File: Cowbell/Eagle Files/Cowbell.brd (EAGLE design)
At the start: 100 x 50 mm, 71 parts, among them IC1 LM741P, Q1 2N3906, T1 2N3904, T2 2N3904, T3 2N3904, T4 2N3904, T5 2N3904, T6 2N3904, T7 2N3904, T8 2N3904

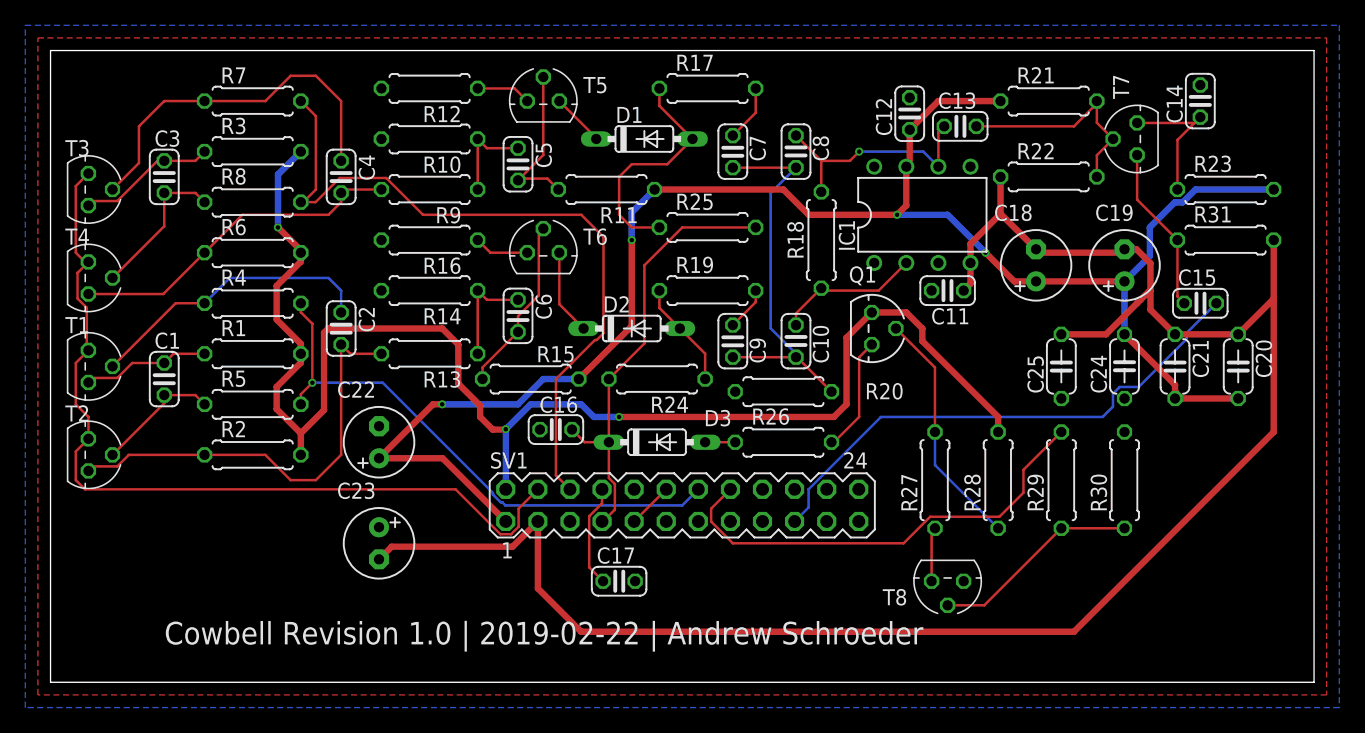
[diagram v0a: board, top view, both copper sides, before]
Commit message: cleanup
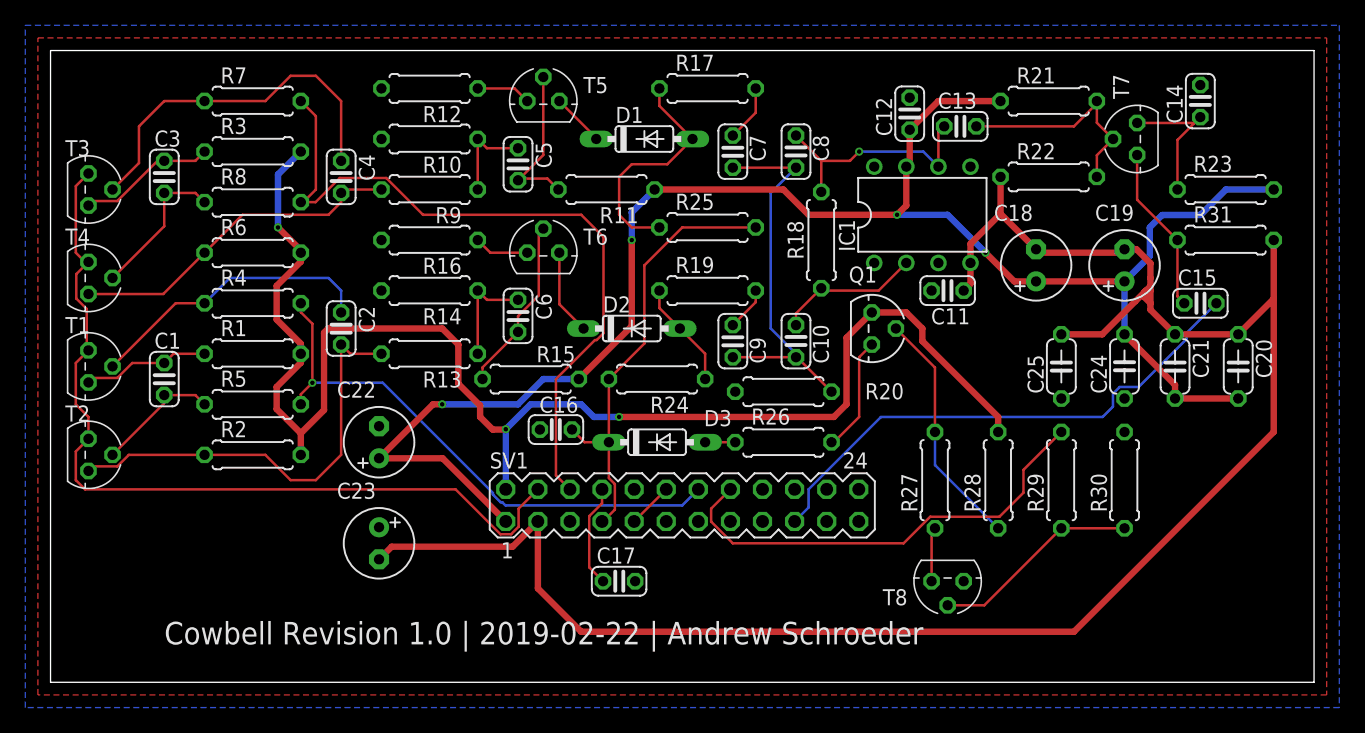
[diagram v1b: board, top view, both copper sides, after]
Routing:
- net -12V: track 148.5 -> 150.2 mm
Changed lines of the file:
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@@
 <?xml version="1.0" encoding="utf-8"?>
 <!DOCTYPE eagle SYSTEM "eagle.dtd">
-<eagle version="9.2.2">
+<eagle version="9.3.1">
 <drawing>
 <settings>
@@
 </class>
 </classes>
-<designrules name="JLCPCB2Layer">
+<designrules name="SeeedStudio_2layer_DRU_no_angle_20140221">
 <description language="de">&lt;b&gt;EAGLE Design Rules&lt;/b&gt;
 &lt;p&gt;
@@
 </description>
 <param name="layerSetup" value="(1*16)"/>
-<param name="mtCopper" value="0.035mm 0.035mm 0.035mm 0.035mm 0.035mm 0.035mm 0.035mm 0.035mm 0.035mm 0.035mm 0.035mm 0.035mm 0.035mm 0.035mm 0.035mm 0.035mm"/>
-<param name="mtIsolate" value="1.5mm 0.15mm 0.2mm 0.15mm 0.2mm 0.15mm 0.2mm 0.15mm 0.2mm 0.15mm 0.2mm 0.15mm 0.2mm 0.15mm 0.2mm"/>
+<param name="mtCopper" value="0.035mm 0.0175mm 0.035mm 0.035mm 0.035mm 0.035mm 0.035mm 0.035mm 0.035mm 0.035mm 0.035mm 0.035mm 0.035mm 0.035mm 0.0175mm 0.035mm"/>
+<param name="mtIsolate" value="1.5mm 1.1mm 0.2mm 0.15mm 0.2mm 0.15mm 0.2mm 0.15mm 0.2mm 0.15mm 0.2mm 0.15mm 0.2mm 0.15mm 0.2mm"/>
 <param name="mdWireWire" value="6mil"/>
 <param name="mdWirePad" value="6mil"/>
@@
 <param name="mdSmdStop" value="0mil"/>
 <param name="msWidth" value="6mil"/>
-<param name="msDrill" value="10mil"/>
-<param name="msMicroVia" value="10mil"/>
+<param name="msDrill" value="12mil"/>
+<param name="msMicroVia" value="12mil"/>
 <param name="msBlindViaRatio" value="0.5"/>
 <param name="rvPadTop" value="0.25"/>
@@
 <param name="rvMicroViaOuter" value="0.25"/>
 <param name="rvMicroViaInner" value="0.25"/>
-<param name="rlMinPadTop" value="6mil"/>
+<param name="rlMinPadTop" value="10mil"/>
 <param name="rlMaxPadTop" value="20mil"/>
-<param name="rlMinPadInner" value="6mil"/>
+<param name="rlMinPadInner" value="10mil"/>
 <param name="rlMaxPadInner" value="20mil"/>
-<param name="rlMinPadBottom" value="6mil"/>
+<param name="rlMinPadBottom" value="10mil"/>
 <param name="rlMaxPadBottom" value="20mil"/>
 <param name="rlMinViaOuter" value="6mil"/>
@@
 <wire x1="46" y1="37.19" x2="47.81" y2="39" width="0.508" layer="16"/>
 <wire x1="85" y1="31.73" x2="85" y2="27.54" width="0.508" layer="16"/>
-<wire x1="90.62684375" y1="39" x2="96.81" y2="39" width="0.508" layer="16"/>
+<wire x1="93.02684375" y1="39" x2="96.81" y2="39" width="0.508" layer="16"/>
 <wire x1="31.03" y1="17.73" x2="36.03" y2="12.73" width="0.508" layer="1"/>
 <wire x1="31.03" y1="17.73" x2="26" y2="17.73" width="0.508" layer="1"/>
@@
 <wire x1="85" y1="31.73" x2="87" y2="33.73" width="0.508" layer="16"/>
 <wire x1="87" y1="33.73" x2="87" y2="36" width="0.508" layer="16"/>
-<wire x1="87" y1="36" x2="88.984" y2="37.984" width="0.508" layer="16"/>
-<wire x1="88.984" y1="37.984" x2="89.61084375" y2="37.984" width="0.508" layer="16"/>
-<wire x1="89.61084375" y1="37.984" x2="90.62684375" y2="39" width="0.508" layer="16"/>
+<wire x1="87" y1="36" x2="87.984" y2="36.984" width="0.508" layer="16"/>
+<wire x1="87.984" y1="36.984" x2="91.01084375" y2="36.984" width="0.508" layer="16"/>
+<wire x1="91.01084375" y1="36.984" x2="93.02684375" y2="39" width="0.508" layer="16"/>
 </signal>
 <signal name="-12V">
@@
 <wire x1="89" y1="27.54" x2="87.0525" y2="29.4875" width="0.508" layer="1"/>
 <wire x1="85" y1="34" x2="85" y2="34.27" width="0.2" layer="1"/>
-<wire x1="87.0525" y1="29.4875" x2="87.0525" y2="31" width="0.508" layer="1"/>
-<wire x1="87.0525" y1="31" x2="87.0525" y2="33.1659625" width="0.508" layer="1"/>
+<wire x1="87.0525" y1="29.4875" x2="87.0525" y2="30" width="0.508" layer="1"/>
+<wire x1="87.0525" y1="30" x2="87.0525" y2="31" width="0.508" layer="1"/>
+<wire x1="87.0525" y1="31" x2="87.0525" y2="31.3525" width="0.508" layer="1"/>
+<wire x1="87.0525" y1="32" x2="87.0525" y2="33.1659625" width="0.508" layer="1"/>
 <wire x1="87.0525" y1="33.1659625" x2="85.9484625" y2="34.27" width="0.508" layer="1"/>
 <wire x1="85" y1="34.27" x2="85.9484625" y2="34.27" width="0.508" layer="1"/>
-<wire x1="80" y1="27.54" x2="83.54" y2="27.54" width="0.508" layer="1"/>
-<wire x1="83.54" y1="27.54" x2="86" y2="30" width="0.508" layer="1"/>
-<wire x1="86" y1="30" x2="86.27" y2="30.27" width="0.508" layer="1"/>
+<wire x1="80" y1="27.54" x2="83.24" y2="27.54" width="0.508" layer="1"/>
 <wire x1="75.19" y1="40" x2="75.19" y2="37.08" width="0.508" layer="1"/>
 <wire x1="75.19" y1="37.08" x2="78" y2="34.27" width="0.508" layer="1"/>
@@
 <wire x1="96.81" y1="19.81" x2="96.81" y2="30.35" width="0.508" layer="1"/>
 <wire x1="38.57" y1="7.43" x2="42" y2="4" width="0.508" layer="1"/>
-<wire x1="86.27" y1="30.27" x2="87" y2="31" width="0.508" layer="1"/>
-<wire x1="87" y1="31" x2="87.0525" y2="31" width="0.508" layer="1"/>
+<wire x1="83.24" y1="27.54" x2="85.85" y2="30.15" width="0.508" layer="1"/>
+<wire x1="85.85" y1="30.15" x2="86.55" y2="30.85" width="0.508" layer="1"/>
+<wire x1="86.55" y1="30.85" x2="86.7" y2="31" width="0.508" layer="1"/>
+<wire x1="86.7" y1="31" x2="87.0525" y2="31" width="0.508" layer="1"/>
+<wire x1="87.0525" y1="30" x2="86.55" y2="30.5025" width="0.508" layer="1"/>
+<wire x1="86.55" y1="30.5025" x2="86.55" y2="30.85" width="0.508" layer="1"/>
+<wire x1="86.55" y1="30.85" x2="87.0525" y2="31.3525" width="0.508" layer="1"/>
+<wire x1="87.0525" y1="31.3525" x2="87.0525" y2="32" width="0.508" layer="1"/>
 </signal>
 <signal name="OUTPUT">
@@
 <wire x1="2" y1="16" x2="2" y2="18.27" width="0.2" layer="1"/>
 <wire x1="2" y1="18.27" x2="3" y2="19.27" width="0.2" layer="1"/>
-<wire x1="2.865" y1="29.64594375" x2="2.865" y2="26.135" width="0.2" layer="1"/>
-<wire x1="2.138" y1="30.37294375" x2="2.865" y2="29.64594375" width="0.2" layer="1"/>
-<wire x1="2.138" y1="32.408" x2="2.138" y2="30.37294375" width="0.2" layer="1"/>
+<wire x1="2.865" y1="29.54594375" x2="2.865" y2="26.135" width="0.2" layer="1"/>
+<wire x1="2.038" y1="30.37294375" x2="2.865" y2="29.54594375" width="0.2" layer="1"/>
+<wire x1="2.038" y1="32.308" x2="2.038" y2="30.37294375" width="0.2" layer="1"/>
 <wire x1="3" y1="33.27" x2="2.865" y2="33.135" width="0.2" layer="1"/>
-<wire x1="2.865" y1="33.135" x2="2.138" y2="32.408" width="0.2" layer="1"/>
+<wire x1="2.865" y1="33.135" x2="2.038" y2="32.308" width="0.2" layer="1"/>
 <wire x1="3" y1="40.27" x2="2" y2="39.27" width="0.2" layer="1"/>
 <wire x1="2" y1="34" x2="2.865" y2="33.135" width="0.2" layer="1"/>
